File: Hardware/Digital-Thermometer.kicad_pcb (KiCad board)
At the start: 2 copper layers, 90.2 x 66 mm, 22 parts, among them Q1 BC547, SW1 SW_Push, U1 Arduino_Nano_v3, U2 DHT11, U3 Display_3461BS

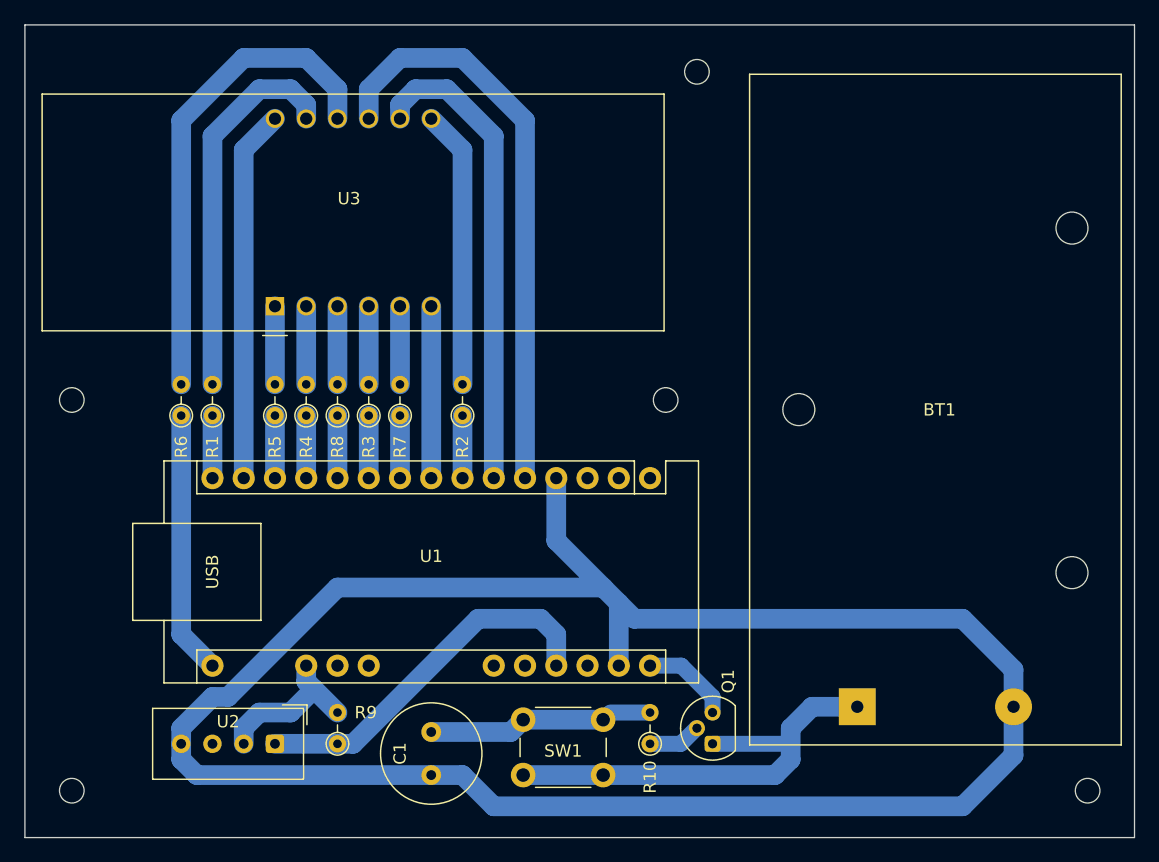
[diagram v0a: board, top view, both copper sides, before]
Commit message: Minor PCB improvements
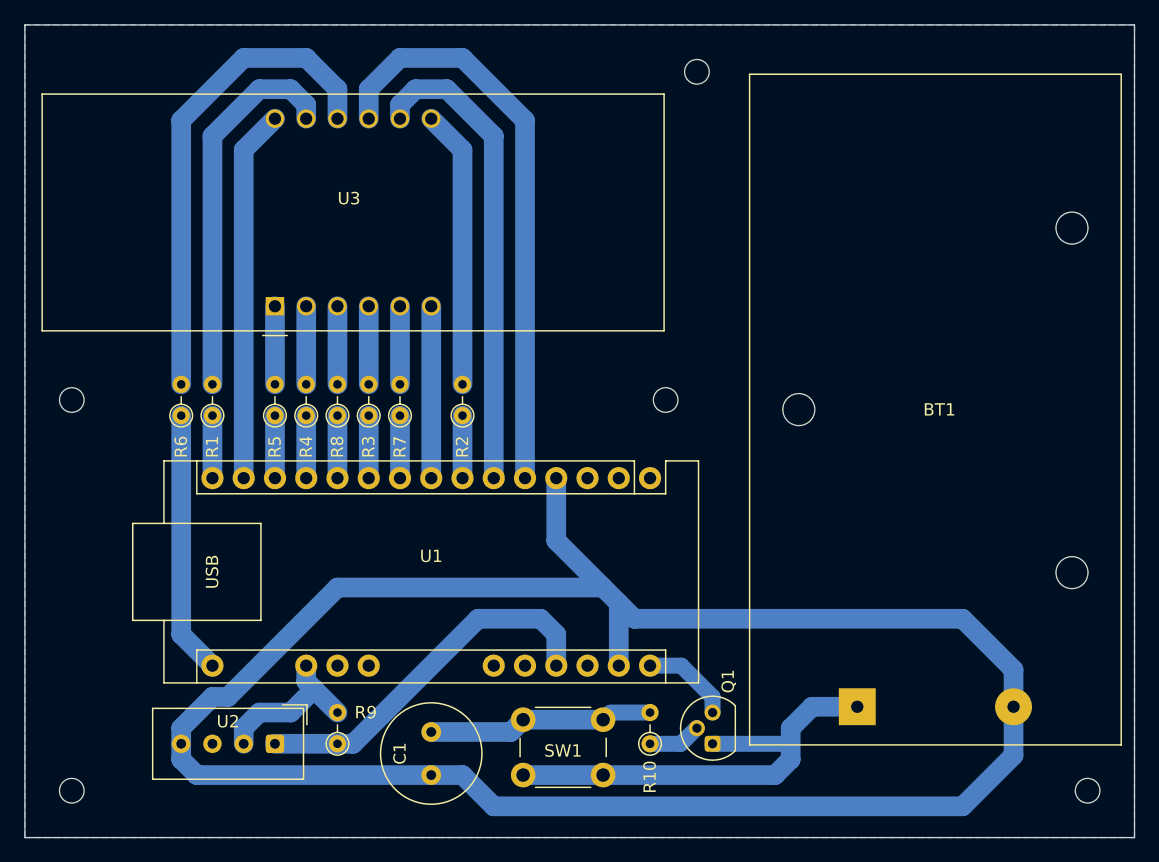
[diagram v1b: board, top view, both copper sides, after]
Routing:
- added copper zone on B.Cu, net GND
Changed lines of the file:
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@@
 		(net 36)
+	)
+	(zone
+		(net 1)
+		(net_name "GND")
+		(layer "B.Cu")
+		(name "GND")
+		(hatch edge 0.5)
+		(connect_pads yes
+			(clearance 1)
+		)
+		(min_thickness 0.25)
+		(filled_areas_thickness no)
+		(fill yes
+			(thermal_gap 0.5)
+			(thermal_bridge_width 0.5)
+			(island_removal_mode 1)
+			(island_area_min 10)
+		)
+		(polygon
+			(pts
+				(xy 127 71.12) (xy 127 137.16) (xy 217.17 137.16) (xy 217.17 71.12)
+			)
+		)
 	)
 	(embedded_fonts no)
